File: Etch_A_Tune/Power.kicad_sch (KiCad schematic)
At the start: 17 parts, among them U4 TPS62063DSGR

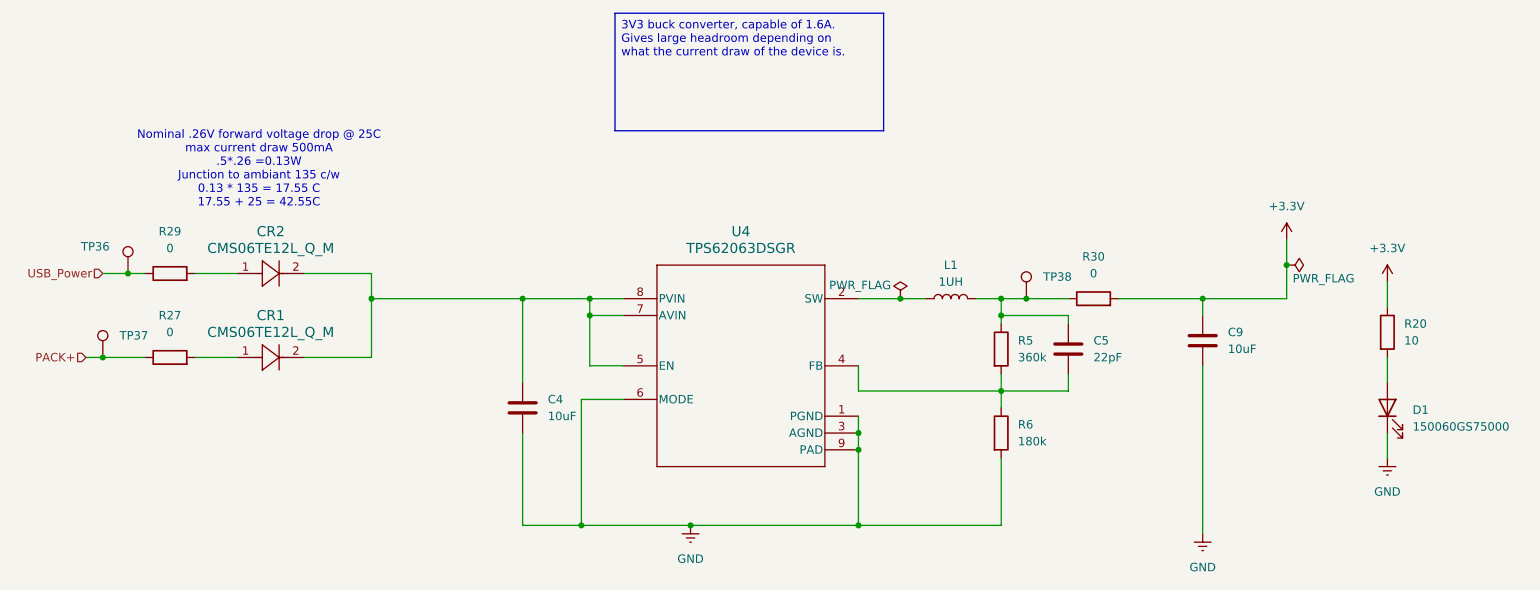
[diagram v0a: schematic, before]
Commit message: Another Update! :D
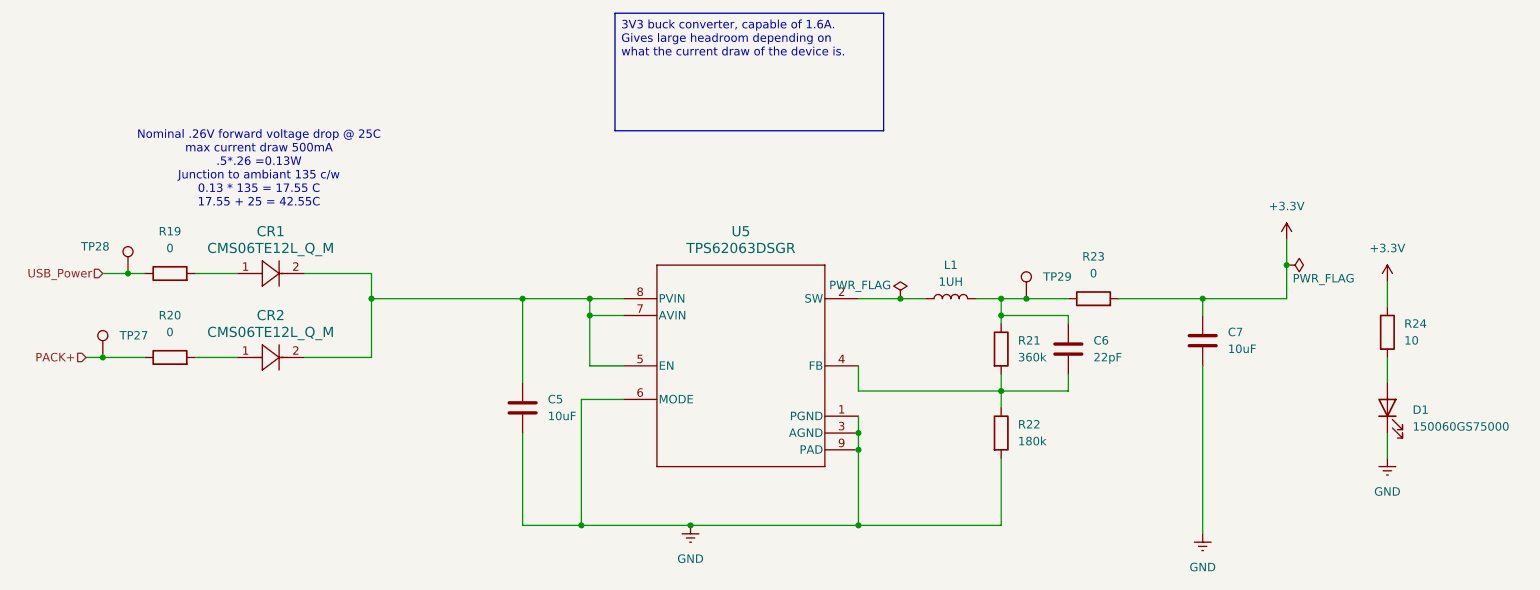
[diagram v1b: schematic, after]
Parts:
- renumbered C4 to C5, C5 to C6, C9 to C7, CR2 to CR1, CR1 to CR2, R29 to R19, R27 to R20, R5 to R21, R6 to R22, R30 to R23, R20 to R24, TP37 to TP27, TP36 to TP28, TP38 to TP29, U4 to U5
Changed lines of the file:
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@@
 		(dnp no)
 		(fields_autoplaced yes)
-		(property "Reference" "CR2"
+		(property "Reference" "CR1"
 			(at 54.61 73.66 0)
 			(effects
@@
 			(project "Etch_A_Tune"
 				(path "/b4cdadf2-c4fe-48fe-ba6a-e15d1cad03b2/e5e22929-d6f1-4829-905c-a53e6965babb"
-					(reference "CR2")
+					(reference "CR1")
 					(unit 1)
 				)
@@
 		(dnp no)
 		(fields_autoplaced yes)
-		(property "Reference" "R6"
+		(property "Reference" "R22"
 			(at 167.64 102.8699 0)
 			(effects
@@
 			(project "Etch_A_Tune"
 				(path "/b4cdadf2-c4fe-48fe-ba6a-e15d1cad03b2/e5e22929-d6f1-4829-905c-a53e6965babb"
-					(reference "R6")
+					(reference "R22")
 					(unit 1)
 				)
@@
 		(dnp no)
 		(fields_autoplaced yes)
-		(property "Reference" "#PWR08"
+		(property "Reference" "#PWR013"
 			(at 118.11 124.46 0)
 			(effects
@@
 			(project "Etch_A_Tune"
 				(path "/b4cdadf2-c4fe-48fe-ba6a-e15d1cad03b2/e5e22929-d6f1-4829-905c-a53e6965babb"
-					(reference "#PWR08")
+					(reference "#PWR013")
 					(unit 1)
 				)
@@
 		(dnp no)
 		(fields_autoplaced yes)
-		(property "Reference" "R5"
+		(property "Reference" "R21"
 			(at 167.64 90.1699 0)
 			(effects
@@
 			(project "Etch_A_Tune"
 				(path "/b4cdadf2-c4fe-48fe-ba6a-e15d1cad03b2/e5e22929-d6f1-4829-905c-a53e6965babb"
-					(reference "R5")
+					(reference "R21")
 					(unit 1)
 				)
@@
 		(dnp no)
 		(fields_autoplaced yes)
-		(property "Reference" "#PWR038"
+		(property "Reference" "#PWR014"
 			(at 195.58 125.73 0)
 			(effects
@@
 			(project "Etch_A_Tune"
 				(path "/b4cdadf2-c4fe-48fe-ba6a-e15d1cad03b2/e5e22929-d6f1-4829-905c-a53e6965babb"
-					(reference "#PWR038")
+					(reference "#PWR014")
 					(unit 1)
 				)
@@
 		(dnp no)
 		(fields_autoplaced yes)
-		(property "Reference" "C5"
+		(property "Reference" "C6"
 			(at 179.07 90.1699 0)
 			(effects
@@
 			(project "Etch_A_Tune"
 				(path "/b4cdadf2-c4fe-48fe-ba6a-e15d1cad03b2/e5e22929-d6f1-4829-905c-a53e6965babb"
-					(reference "C5")
+					(reference "C6")
 					(unit 1)
 				)
@@
 		(dnp no)
 		(fields_autoplaced yes)
-		(property "Reference" "U4"
+		(property "Reference" "U5"
 			(at 125.73 73.66 0)
 			(effects
@@
 			(project ""
 				(path "/b4cdadf2-c4fe-48fe-ba6a-e15d1cad03b2/e5e22929-d6f1-4829-905c-a53e6965babb"
-					(reference "U4")
+					(reference "U5")
 					(unit 1)
 				)
@@
 		(dnp no)
 		(fields_autoplaced yes)
-		(property "Reference" "C4"
+		(property "Reference" "C5"
 			(at 96.52 99.0599 0)
 			(effects
@@
 			(project "Etch_A_Tune"
 				(path "/b4cdadf2-c4fe-48fe-ba6a-e15d1cad03b2/e5e22929-d6f1-4829-905c-a53e6965babb"
-					(reference "C4")
+					(reference "C5")
 					(unit 1)
 				)
@@
 		(dnp no)
 		(fields_autoplaced yes)
-		(property "Reference" "#PWR032"
+		(property "Reference" "#PWR017"
 			(at 223.52 114.3 0)
 			(effects
@@
 			(project "Etch_A_Tune"
 				(path "/b4cdadf2-c4fe-48fe-ba6a-e15d1cad03b2/e5e22929-d6f1-4829-905c-a53e6965babb"
-					(reference "#PWR032")
+					(reference "#PWR017")
 					(unit 1)
 				)
@@
 		(dnp no)
 		(fields_autoplaced yes)
-		(property "Reference" "R29"
+		(property "Reference" "R19"
 			(at 39.37 73.66 90)
 			(effects
@@
 			(project "Etch_A_Tune"
 				(path "/b4cdadf2-c4fe-48fe-ba6a-e15d1cad03b2/e5e22929-d6f1-4829-905c-a53e6965babb"
-					(reference "R29")
+					(reference "R19")
 					(unit 1)
 				)
@@
 		(dnp no)
 		(fields_autoplaced yes)
-		(property "Reference" "CR1"
+		(property "Reference" "CR2"
 			(at 54.61 86.36 0)
 			(effects
@@
 			(project ""
 				(path "/b4cdadf2-c4fe-48fe-ba6a-e15d1cad03b2/e5e22929-d6f1-4829-905c-a53e6965babb"
-					(reference "CR1")
+					(reference "CR2")
 					(unit 1)
 				)
@@
 		(dnp no)
 		(fields_autoplaced yes)
-		(property "Reference" "#PWR09"
+		(property "Reference" "#PWR015"
 			(at 208.28 78.74 0)
 			(effects
@@
 			(project "Etch_A_Tune"
 				(path "/b4cdadf2-c4fe-48fe-ba6a-e15d1cad03b2/e5e22929-d6f1-4829-905c-a53e6965babb"
-					(reference "#PWR09")
+					(reference "#PWR015")
 					(unit 1)
 				)
@@
 		(on_board yes)
 		(dnp no)
-		(property "Reference" "#FLG03"
+		(property "Reference" "#FLG04"
 			(at 149.86 81.915 0)
 			(effects
@@
 			(project "Etch_A_Tune"
 				(path "/b4cdadf2-c4fe-48fe-ba6a-e15d1cad03b2/e5e22929-d6f1-4829-905c-a53e6965babb"
-					(reference "#FLG03")
+					(reference "#FLG04")
 					(unit 1)
 				)
@@
 		(dnp no)
 		(fields_autoplaced yes)
-		(property "Reference" "C9"
+		(property "Reference" "C7"
 			(at 199.39 88.8999 0)
 			(effects
@@
 			(project "Etch_A_Tune"
 				(path "/b4cdadf2-c4fe-48fe-ba6a-e15d1cad03b2/e5e22929-d6f1-4829-905c-a53e6965babb"
-					(reference "C9")
+					(reference "C7")
 					(unit 1)
 				)
@@
 		(dnp no)
 		(fields_autoplaced yes)
-		(property "Reference" "R27"
+		(property "Reference" "R20"
 			(at 39.37 86.36 90)
 			(effects
@@
 			(project "Etch_A_Tune"
 				(path "/b4cdadf2-c4fe-48fe-ba6a-e15d1cad03b2/e5e22929-d6f1-4829-905c-a53e6965babb"
-					(reference "R27")
+					(reference "R20")
 					(unit 1)
 				)
@@
 		(dnp no)
 		(fields_autoplaced yes)
-		(property "Reference" "TP38"
+		(property "Reference" "TP29"
 			(at 171.45 80.5179 0)
 			(effects
@@
 			(project "Etch_A_Tune"
 				(path "/b4cdadf2-c4fe-48fe-ba6a-e15d1cad03b2/e5e22929-d6f1-4829-905c-a53e6965babb"
-					(reference "TP38")
+					(reference "TP29")
 					(unit 1)
 				)
@@
 		(dnp no)
 		(fields_autoplaced yes)
-		(property "Reference" "R20"
+		(property "Reference" "R24"
 			(at 226.06 87.6299 0)
 			(effects
@@
 			(project "Etch_A_Tune"
 				(path "/b4cdadf2-c4fe-48fe-ba6a-e15d1cad03b2/e5e22929-d6f1-4829-905c-a53e6965babb"
-					(reference "R20")
+					(reference "R24")
 					(unit 1)
 				)
@@
 		(dnp no)
 		(fields_autoplaced yes)
-		(property "Reference" "R30"
+		(property "Reference" "R23"
 			(at 179.07 77.47 90)
 			(effects
@@
 			(project "Etch_A_Tune"
 				(path "/b4cdadf2-c4fe-48fe-ba6a-e15d1cad03b2/e5e22929-d6f1-4829-905c-a53e6965babb"
-					(reference "R30")
+					(reference "R23")
 					(unit 1)
 				)
@@
 		(dnp no)
 		(fields_autoplaced yes)
-		(property "Reference" "#PWR06"
+		(property "Reference" "#PWR016"
 			(at 223.52 85.09 0)
 			(effects
@@
 			(project "Etch_A_Tune"
 				(path "/b4cdadf2-c4fe-48fe-ba6a-e15d1cad03b2/e5e22929-d6f1-4829-905c-a53e6965babb"
-					(reference "#PWR06")
+					(reference "#PWR016")
 					(unit 1)
 				)
@@
 		(on_board yes)
 		(dnp no)
-		(property "Reference" "TP36"
+		(property "Reference" "TP28"
 			(at 25.908 75.946 0)
 			(effects
@@
 			(project "Etch_A_Tune"
 				(path "/b4cdadf2-c4fe-48fe-ba6a-e15d1cad03b2/e5e22929-d6f1-4829-905c-a53e6965babb"
-					(reference "TP36")
+					(reference "TP28")
 					(unit 1)
 				)
@@
 		(dnp no)
 		(fields_autoplaced yes)
-		(property "Reference" "TP37"
+		(property "Reference" "TP27"
 			(at 31.75 89.4079 0)
 			(effects
@@
 			(project "Etch_A_Tune"
 				(path "/b4cdadf2-c4fe-48fe-ba6a-e15d1cad03b2/e5e22929-d6f1-4829-905c-a53e6965babb"
-					(reference "TP37")
-					(unit 1)
-				)
+					(reference "TP27")
+					(unit 1)
+				)

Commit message: pdf docs
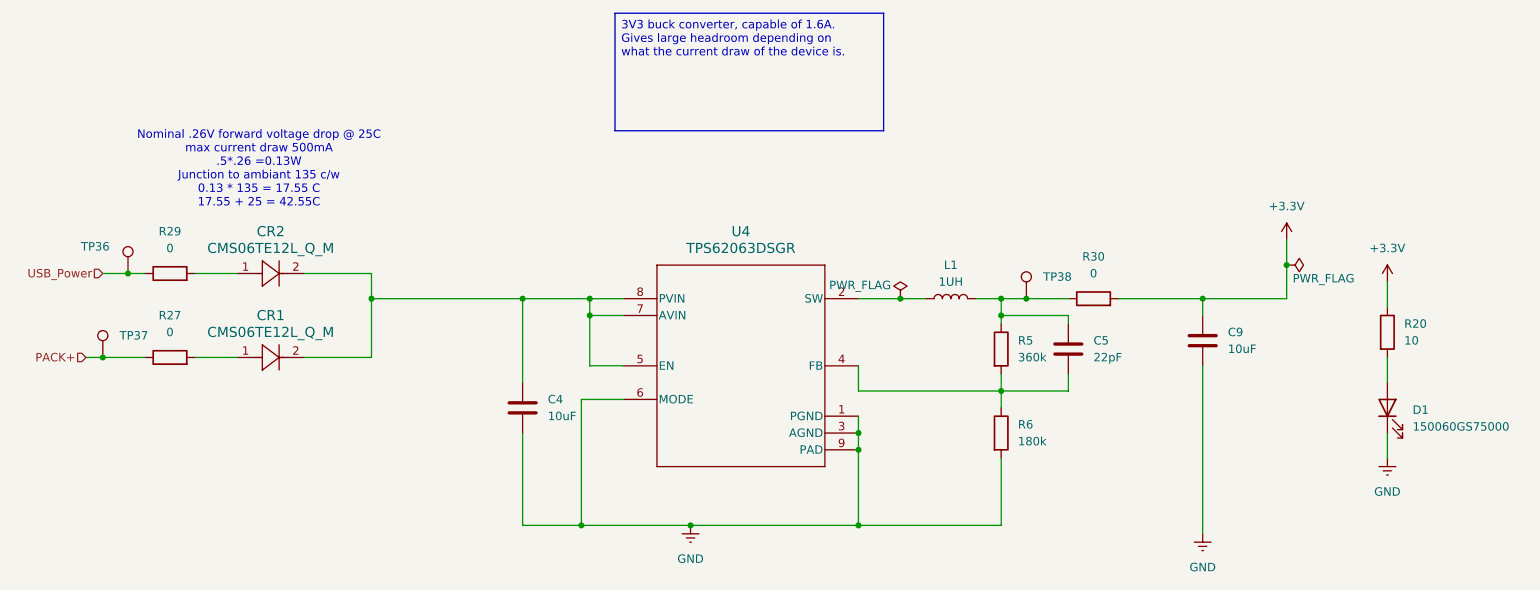
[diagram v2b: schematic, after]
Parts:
- renumbered C5 to C4, C6 to C5, C7 to C9, CR2 to CR1, CR1 to CR2, R24 to R20, R20 to R27, R19 to R29, R23 to R30, R21 to R5, R22 to R6, TP28 to TP36, TP27 to TP37, TP29 to TP38, U5 to U4
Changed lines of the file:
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@@
 		(dnp no)
 		(fields_autoplaced yes)
-		(property "Reference" "CR1"
+		(property "Reference" "CR2"
 			(at 54.61 73.66 0)
 			(effects
@@
 			(project "Etch_A_Tune"
 				(path "/b4cdadf2-c4fe-48fe-ba6a-e15d1cad03b2/e5e22929-d6f1-4829-905c-a53e6965babb"
-					(reference "CR1")
+					(reference "CR2")
 					(unit 1)
 				)
@@
 		(dnp no)
 		(fields_autoplaced yes)
-		(property "Reference" "R22"
+		(property "Reference" "R6"
 			(at 167.64 102.8699 0)
 			(effects
@@
 			(project "Etch_A_Tune"
 				(path "/b4cdadf2-c4fe-48fe-ba6a-e15d1cad03b2/e5e22929-d6f1-4829-905c-a53e6965babb"
-					(reference "R22")
+					(reference "R6")
 					(unit 1)
 				)
@@
 		(dnp no)
 		(fields_autoplaced yes)
-		(property "Reference" "#PWR013"
+		(property "Reference" "#PWR08"
 			(at 118.11 124.46 0)
 			(effects
@@
 			(project "Etch_A_Tune"
 				(path "/b4cdadf2-c4fe-48fe-ba6a-e15d1cad03b2/e5e22929-d6f1-4829-905c-a53e6965babb"
-					(reference "#PWR013")
+					(reference "#PWR08")
 					(unit 1)
 				)
@@
 		(dnp no)
 		(fields_autoplaced yes)
-		(property "Reference" "R21"
+		(property "Reference" "R5"
 			(at 167.64 90.1699 0)
 			(effects
@@
 			(project "Etch_A_Tune"
 				(path "/b4cdadf2-c4fe-48fe-ba6a-e15d1cad03b2/e5e22929-d6f1-4829-905c-a53e6965babb"
-					(reference "R21")
+					(reference "R5")
 					(unit 1)
 				)
@@
 		(dnp no)
 		(fields_autoplaced yes)
-		(property "Reference" "#PWR014"
+		(property "Reference" "#PWR038"
 			(at 195.58 125.73 0)
 			(effects
@@
 			(project "Etch_A_Tune"
 				(path "/b4cdadf2-c4fe-48fe-ba6a-e15d1cad03b2/e5e22929-d6f1-4829-905c-a53e6965babb"
-					(reference "#PWR014")
+					(reference "#PWR038")
 					(unit 1)
 				)
@@
 		(dnp no)
 		(fields_autoplaced yes)
-		(property "Reference" "C6"
+		(property "Reference" "C5"
 			(at 179.07 90.1699 0)
 			(effects
@@
 			(project "Etch_A_Tune"
 				(path "/b4cdadf2-c4fe-48fe-ba6a-e15d1cad03b2/e5e22929-d6f1-4829-905c-a53e6965babb"
-					(reference "C6")
+					(reference "C5")
 					(unit 1)
 				)
@@
 		(dnp no)
 		(fields_autoplaced yes)
-		(property "Reference" "U5"
+		(property "Reference" "U4"
 			(at 125.73 73.66 0)
 			(effects
@@
 			(project ""
 				(path "/b4cdadf2-c4fe-48fe-ba6a-e15d1cad03b2/e5e22929-d6f1-4829-905c-a53e6965babb"
-					(reference "U5")
+					(reference "U4")
 					(unit 1)
 				)
@@
 		(dnp no)
 		(fields_autoplaced yes)
-		(property "Reference" "C5"
+		(property "Reference" "C4"
 			(at 96.52 99.0599 0)
 			(effects
@@
 			(project "Etch_A_Tune"
 				(path "/b4cdadf2-c4fe-48fe-ba6a-e15d1cad03b2/e5e22929-d6f1-4829-905c-a53e6965babb"
-					(reference "C5")
+					(reference "C4")
 					(unit 1)
 				)
@@
 		(dnp no)
 		(fields_autoplaced yes)
-		(property "Reference" "#PWR017"
+		(property "Reference" "#PWR032"
 			(at 223.52 114.3 0)
 			(effects
@@
 			(project "Etch_A_Tune"
 				(path "/b4cdadf2-c4fe-48fe-ba6a-e15d1cad03b2/e5e22929-d6f1-4829-905c-a53e6965babb"
-					(reference "#PWR017")
+					(reference "#PWR032")
 					(unit 1)
 				)
@@
 		(dnp no)
 		(fields_autoplaced yes)
-		(property "Reference" "R19"
+		(property "Reference" "R29"
 			(at 39.37 73.66 90)
 			(effects
@@
 			(project "Etch_A_Tune"
 				(path "/b4cdadf2-c4fe-48fe-ba6a-e15d1cad03b2/e5e22929-d6f1-4829-905c-a53e6965babb"
-					(reference "R19")
+					(reference "R29")
 					(unit 1)
 				)
@@
 		(dnp no)
 		(fields_autoplaced yes)
-		(property "Reference" "CR2"
+		(property "Reference" "CR1"
 			(at 54.61 86.36 0)
 			(effects
@@
 			(project ""
 				(path "/b4cdadf2-c4fe-48fe-ba6a-e15d1cad03b2/e5e22929-d6f1-4829-905c-a53e6965babb"
-					(reference "CR2")
+					(reference "CR1")
 					(unit 1)
 				)
@@
 		(dnp no)
 		(fields_autoplaced yes)
-		(property "Reference" "#PWR015"
+		(property "Reference" "#PWR09"
 			(at 208.28 78.74 0)
 			(effects
@@
 			(project "Etch_A_Tune"
 				(path "/b4cdadf2-c4fe-48fe-ba6a-e15d1cad03b2/e5e22929-d6f1-4829-905c-a53e6965babb"
-					(reference "#PWR015")
+					(reference "#PWR09")
 					(unit 1)
 				)
@@
 		(on_board yes)
 		(dnp no)
-		(property "Reference" "#FLG04"
+		(property "Reference" "#FLG03"
 			(at 149.86 81.915 0)
 			(effects
@@
 			(project "Etch_A_Tune"
 				(path "/b4cdadf2-c4fe-48fe-ba6a-e15d1cad03b2/e5e22929-d6f1-4829-905c-a53e6965babb"
-					(reference "#FLG04")
+					(reference "#FLG03")
 					(unit 1)
 				)
@@
 		(dnp no)
 		(fields_autoplaced yes)
-		(property "Reference" "C7"
+		(property "Reference" "C9"
 			(at 199.39 88.8999 0)
 			(effects
@@
 			(project "Etch_A_Tune"
 				(path "/b4cdadf2-c4fe-48fe-ba6a-e15d1cad03b2/e5e22929-d6f1-4829-905c-a53e6965babb"
-					(reference "C7")
+					(reference "C9")
 					(unit 1)
 				)
@@
 		(dnp no)
 		(fields_autoplaced yes)
-		(property "Reference" "R20"
+		(property "Reference" "R27"
 			(at 39.37 86.36 90)
 			(effects
@@
 			(project "Etch_A_Tune"
 				(path "/b4cdadf2-c4fe-48fe-ba6a-e15d1cad03b2/e5e22929-d6f1-4829-905c-a53e6965babb"
-					(reference "R20")
+					(reference "R27")
 					(unit 1)
 				)
@@
 		(dnp no)
 		(fields_autoplaced yes)
-		(property "Reference" "TP29"
+		(property "Reference" "TP38"
 			(at 171.45 80.5179 0)
 			(effects
@@
 			(project "Etch_A_Tune"
 				(path "/b4cdadf2-c4fe-48fe-ba6a-e15d1cad03b2/e5e22929-d6f1-4829-905c-a53e6965babb"
-					(reference "TP29")
+					(reference "TP38")
 					(unit 1)
 				)
@@
 		(dnp no)
 		(fields_autoplaced yes)
-		(property "Reference" "R24"
+		(property "Reference" "R20"
 			(at 226.06 87.6299 0)
 			(effects
@@
 			(project "Etch_A_Tune"
 				(path "/b4cdadf2-c4fe-48fe-ba6a-e15d1cad03b2/e5e22929-d6f1-4829-905c-a53e6965babb"
-					(reference "R24")
+					(reference "R20")
 					(unit 1)
 				)
@@
 		(dnp no)
 		(fields_autoplaced yes)
-		(property "Reference" "R23"
+		(property "Reference" "R30"
 			(at 179.07 77.47 90)
 			(effects
@@
 			(project "Etch_A_Tune"
 				(path "/b4cdadf2-c4fe-48fe-ba6a-e15d1cad03b2/e5e22929-d6f1-4829-905c-a53e6965babb"
-					(reference "R23")
+					(reference "R30")
 					(unit 1)
 				)
@@
 		(dnp no)
 		(fields_autoplaced yes)
-		(property "Reference" "#PWR016"
+		(property "Reference" "#PWR06"
 			(at 223.52 85.09 0)
 			(effects
@@
 			(project "Etch_A_Tune"
 				(path "/b4cdadf2-c4fe-48fe-ba6a-e15d1cad03b2/e5e22929-d6f1-4829-905c-a53e6965babb"
-					(reference "#PWR016")
+					(reference "#PWR06")
 					(unit 1)
 				)
@@
 		(on_board yes)
 		(dnp no)
-		(property "Reference" "TP28"
+		(property "Reference" "TP36"
 			(at 25.908 75.946 0)
 			(effects
@@
 			(project "Etch_A_Tune"
 				(path "/b4cdadf2-c4fe-48fe-ba6a-e15d1cad03b2/e5e22929-d6f1-4829-905c-a53e6965babb"
-					(reference "TP28")
+					(reference "TP36")
 					(unit 1)
 				)
@@
 		(dnp no)
 		(fields_autoplaced yes)
-		(property "Reference" "TP27"
+		(property "Reference" "TP37"
 			(at 31.75 89.4079 0)
 			(effects
@@
 			(project "Etch_A_Tune"
 				(path "/b4cdadf2-c4fe-48fe-ba6a-e15d1cad03b2/e5e22929-d6f1-4829-905c-a53e6965babb"
-					(reference "TP27")
-					(unit 1)
-				)
+					(reference "TP37")
+					(unit 1)
+				)
